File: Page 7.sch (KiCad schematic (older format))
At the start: 7 parts, among them U3 MCP7940N-xSN, Y801 32.7680 kHz

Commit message: Updating Page Numbering
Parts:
- removed R801: 10k0, Resistor_SMD:R_0603_1608Metric_Pad1.05x0.95mm_HandSolder, symbol Device:R
- renumbered C801 to C701, C802 to C702, C803 to C703, Y801 to Y701
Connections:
- wire segments 32 -> 28
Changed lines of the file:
@@
 $Descr A4 11693 8268
 encoding utf-8
-Sheet 9 9
+Sheet 8 9
 Title ""
 Date ""
@@
 AR Path="/5EAC05C2/5EB307E0" Ref="C?"  Part="1"
 AR Path="/5ECF32A9/5EB307E0" Ref="C?"  Part="1"
-AR Path="/5ECF31FF/5EB307E0" Ref="C803"  Part="1"
-F 0 "C803" V 7000 3700 50  0000 C CNN
+AR Path="/5ECF31FF/5EB307E0" Ref="C703"  Part="1"
+F 0 "C703" V 7000 3700 50  0000 C CNN
 F 1 "10pF" V 7300 3700 50  0000 C CNN
 F 2 "Capacitor_SMD:C_0603_1608Metric_Pad1.05x0.95mm_HandSolder" H 7188 3550 50  0001 C CNN
@@
 AR Path="/5EAC05C2/5EB307E8" Ref="C?"  Part="1"
 AR Path="/5ECF32A9/5EB307E8" Ref="C?"  Part="1"
-AR Path="/5ECF31FF/5EB307E8" Ref="C802"  Part="1"
-F 0 "C802" V 7000 4300 50  0000 C CNN
+AR Path="/5ECF31FF/5EB307E8" Ref="C702"  Part="1"
+F 0 "C702" V 7000 4300 50  0000 C CNN
 F 1 "10pF" V 7300 4300 50  0000 C CNN
 F 2 "Capacitor_SMD:C_0603_1608Metric_Pad1.05x0.95mm_HandSolder" H 7188 4150 50  0001 C CNN
@@
 AR Path="/5EAC05C2/5EB307EE" Ref="Y?"  Part="1"
 AR Path="/5ECF32A9/5EB307EE" Ref="Y?"  Part="1"
-AR Path="/5ECF31FF/5EB307EE" Ref="Y801"  Part="1"
-F 0 "Y801" H 6550 3850 50  0000 L CNN
+AR Path="/5ECF31FF/5EB307EE" Ref="Y701"  Part="1"
+F 0 "Y701" H 6550 3850 50  0000 L CNN
 F 1 "32.7680 kHz" H 6400 4150 50  0000 L CNN
 F 2 "Name Plate Class Project:Oscillator_MC-405_32.7680K-D__ROHS" H 6550 3700 50  0001 L BNN
@@
 	-1   0    0    1
 $EndComp
-Wire Wire Line
-	5500 4100 5300 4100
-Text Label 4950 4100 0    50   ~ 0
-RTC_INT
 Text Notes 5300 5050 0    98   ~ 20
 Real Time Clock
-Connection ~ 5300 4100
-Wire Wire Line
-	5300 4100 4950 4100
-$Comp
-L Device:R R?
-U 1 1 5EB30819
-P 5300 3050
-AR Path="/5EAC05C2/5EB30819" Ref="R?"  Part="1"
-AR Path="/5ECF32A9/5EB30819" Ref="R?"  Part="1"
-AR Path="/5ECF31FF/5EB30819" Ref="R801"  Part="1"
-F 0 "R801" H 5370 3096 50  0000 L CNN
-F 1 "10k0" H 5370 3005 50  0000 L CNN
-F 2 "Resistor_SMD:R_0603_1608Metric_Pad1.05x0.95mm_HandSolder" V 5230 3050 50  0001 C CNN
-F 3 "~" H 5300 3050 50  0001 C CNN
-	1    5300 3050
-	1    0    0    -1
-$EndComp
 $Comp
 L Device:C C?
@@
 AR Path="/5EAC05C2/5EB30820" Ref="C?"  Part="1"
 AR Path="/5ECF32A9/5EB30820" Ref="C?"  Part="1"
-AR Path="/5ECF31FF/5EB30820" Ref="C801"  Part="1"
-F 0 "C801" H 4150 3150 50  0000 L CNN
+AR Path="/5ECF31FF/5EB30820" Ref="C701"  Part="1"
+F 0 "C701" H 4150 3150 50  0000 L CNN
 F 1 "0.1uF" H 4150 3050 50  0000 L CNN
 F 2 "Capacitor_SMD:C_0603_1608Metric_Pad1.05x0.95mm_HandSolder" H 4538 2950 50  0001 C CNN
@@
 $EndComp
 Wire Wire Line
-	5300 2900 5300 2800
-Connection ~ 5300 2800
-Wire Wire Line
 	5150 3450 5650 3450
 Wire Wire Line
@@
 Wire Wire Line
 	5900 3600 5900 2800
-Wire Wire Line
-	5300 2800 5900 2800
-Wire Wire Line
-	5300 3200 5300 4100
-Wire Wire Line
-	4500 2800 5300 2800
 Connection ~ 4500 2800
 Wire Wire Line
@@
 Text HLabel 4950 4100 0    50   Input ~ 0
 RTC_INT
+Wire Wire Line
+	4500 2800 5900 2800
+Wire Wire Line
+	4950 4100 5500 4100
 $EndSCHEMATC

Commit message: Updates to schematic
Switching to ATMega34UF chip.
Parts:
- B801: Mftr Part No. (none) -> BK-883
- C701: DigiKey Part No. (none) -> 311-1335-1-ND; Manufacturer (none) -> Yageo; Mftr Part No. Yageo CC0603KPX7R7BB104 -> CC0603KPX7R7BB104
- C702, C703: Manufacturer (none) -> Kemet; Mftr Part No. Kemet C0603C100J1GACTU -> C0603C100J1GACTU
- U701: renamed from U3; DigiKey Part No. (none) -> MCP79400-I/SN-ND; Manufacturer (none) -> Microchip; Mftr Part No. (none) -> MCP79400-I/SN
- Y701: DigiKey Part No. (none) -> SER4311TR-ND; Manufacturer (none) -> Epson; Mftr Part No. (none) -> MC-405 32.7680K-E3: ROHS
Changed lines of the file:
@@
 F 1 "10pF" V 7300 3700 50  0000 C CNN
 F 2 "Capacitor_SMD:C_0603_1608Metric_Pad1.05x0.95mm_HandSolder" H 7188 3550 50  0001 C CNN
-F 3 "~" H 7150 3700 50  0001 C CNN
+F 3 "https://content.kemet.com/datasheets/KEM_C1003_C0G_SMD.pdf" H 7150 3700 50  0001 C CNN
 F 4 "399-7816-1-ND" H 7150 3700 50  0001 C CNN "DigiKey Part No."
-F 5 "Kemet C0603C100J1GACTU" H 7150 3700 50  0001 C CNN "Mftr Part No."
+F 5 "C0603C100J1GACTU" H 7150 3700 50  0001 C CNN "Mftr Part No."
+F 6 "Kemet" H 7150 3700 50  0001 C CNN "Manufacturer"
 	1    7150 3700
 	0    1    1    0
@@
 F 1 "10pF" V 7300 4300 50  0000 C CNN
 F 2 "Capacitor_SMD:C_0603_1608Metric_Pad1.05x0.95mm_HandSolder" H 7188 4150 50  0001 C CNN
-F 3 "~" H 7150 4300 50  0001 C CNN
+F 3 "https://content.kemet.com/datasheets/KEM_C1003_C0G_SMD.pdf" H 7150 4300 50  0001 C CNN
 F 4 "399-7816-1-ND" H 7150 4300 50  0001 C CNN "DigiKey Part No."
-F 5 "Kemet C0603C100J1GACTU" H 7150 4300 50  0001 C CNN "Mftr Part No."
+F 5 "C0603C100J1GACTU" H 7150 4300 50  0001 C CNN "Mftr Part No."
+F 6 "Kemet" H 7150 4300 50  0001 C CNN "Manufacturer"
 	1    7150 4300
 	0    1    1    0
@@
 F 2 "Name Plate Class Project:Oscillator_MC-405_32.7680K-D__ROHS" H 6550 3700 50  0001 L BNN
 F 3 "https://support.epson.biz/td/api/doc_check.php?dl=brief_MC-405&lang=en" H 6550 3600 50  0001 L BNN
+F 4 "SER4311TR-ND" H 6650 4000 50  0001 C CNN "DigiKey Part No."
+F 5 "Epson " H 6650 4000 50  0001 C CNN "Manufacturer"
+F 6 "MC-405 32.7680K-E3: ROHS" H 6650 4000 50  0001 C CNN "Mftr Part No."
 	1    6650 4000
 	0    1    1    0
@@
 F 4 "MPD" H 4700 3150 50  0001 L BNN "Field4"
 F 5 "L" H 4700 3050 50  0001 L BNN "Field5"
-F 6 "" H 4850 3450 50  0001 C CNN "Mftr Part No."
+F 6 "BK-883" H 4850 3450 50  0001 C CNN "Mftr Part No."
 F 7 "BK-883-ND" H 4850 3450 50  0001 C CNN "DigiKey Part No."
 F 8 "MPD" H 4850 3450 50  0001 C CNN "Manufacturer"
@@
 F 2 "Capacitor_SMD:C_0603_1608Metric_Pad1.05x0.95mm_HandSolder" H 4538 2950 50  0001 C CNN
 F 3 "https://www.yageo.com/upload/media/product/productsearch/datasheet/mlcc/UPY-GPHC_X7R_6.3V-to-50V_18.pdf" H 4500 3100 50  0001 C CNN
-F 4 "Yageo CC0603KPX7R7BB104" H 4500 3100 50  0001 C CNN "Mftr Part No."
+F 4 "CC0603KPX7R7BB104" H 4500 3100 50  0001 C CNN "Mftr Part No."
+F 5 "Yageo" H 4500 3100 50  0001 C CNN "Manufacturer"
+F 6 "311-1335-1-ND" H 4500 3100 50  0001 C CNN "DigiKey Part No."
 	1    4500 3100
 	1    0    0    -1
@@
 AR Path="/5EAC05C2/5EB307D8" Ref="U?"  Part="1"
 AR Path="/5ECF32A9/5EB307D8" Ref="U?"  Part="1"
-AR Path="/5ECF31FF/5EB307D8" Ref="U3"  Part="1"
-F 0 "U3" H 6000 3600 50  0000 L BNN
+AR Path="/5ECF31FF/5EB307D8" Ref="U701"  Part="1"
+F 0 "U701" H 6000 3600 50  0000 L BNN
 F 1 "MCP7940N-xSN" H 6000 3500 50  0000 L BNN
 F 2 "Package_SO:SOIC-8_3.9x4.9mm_P1.27mm" H 5900 4000 50  0001 C CNN
 F 3 "http://ww1.microchip.com/downloads/en/DeviceDoc/20005010F.pdf" H 5900 4000 50  0001 C CNN
+F 4 "MCP79400-I/SN-ND" H 5900 4000 50  0001 C CNN "DigiKey Part No."
+F 5 "Microchip" H 5900 4000 50  0001 C CNN "Manufacturer"
+F 6 "MCP79400-I/SN" H 5900 4000 50  0001 C CNN "Mftr Part No."
 	1    5900 4000
 	1    0    0    -1

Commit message: Updates
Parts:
- B701: renamed from B801; footprint Name Plate Class Project:BAT_BK-883 -> Name_Plate_Class_Project:BAT_BK-883; symbol Name~Plate~Class~Library:BK-883 -> Name_Plate_Class_Project:BK-883; Field4 MPD -> (none); Field5 L -> (none)
- Y701: footprint Name Plate Class Project:Oscillator_MC-405_32.7680K-D__ROHS -> Name_Plate_Class_Project:Oscillator_MC-405_32.7680K-D__ROHS; symbol Name~Plate~Class~Library:Oscillator_MC-405_32.7680K-D__ROHS -> Name_Plate_Class_Project:Oscillator_MC-405_32.7680K-D__ROHS
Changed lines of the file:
@@
 $EndComp
 $Comp
-L Name~Plate~Class~Library:Oscillator_MC-405_32.7680K-D__ROHS Y?
+L Name_Plate_Class_Project:Oscillator_MC-405_32.7680K-D__ROHS Y?
 U 1 1 5EB307EE
 P 6650 4000
@@
 F 0 "Y701" H 6550 3850 50  0000 L CNN
 F 1 "32.7680 kHz" H 6400 4150 50  0000 L CNN
-F 2 "Name Plate Class Project:Oscillator_MC-405_32.7680K-D__ROHS" H 6550 3700 50  0001 L BNN
+F 2 "Name_Plate_Class_Project:Oscillator_MC-405_32.7680K-D__ROHS" H 6550 3700 50  0001 L BNN
 F 3 "https://support.epson.biz/td/api/doc_check.php?dl=brief_MC-405&lang=en" H 6550 3600 50  0001 L BNN
 F 4 "SER4311TR-ND" H 6650 4000 50  0001 C CNN "DigiKey Part No."
@@
 $EndComp
 $Comp
-L Name~Plate~Class~Library:BK-883 B?
+L Name_Plate_Class_Project:BK-883 B?
 U 1 1 5EB3080E
 P 4850 3450
 AR Path="/5EAC05C2/5EB3080E" Ref="B?"  Part="1"
 AR Path="/5ECF32A9/5EB3080E" Ref="B?"  Part="1"
-AR Path="/5ECF31FF/5EB3080E" Ref="B801"  Part="1"
-F 0 "B801" H 4850 3183 50  0000 C CNN
+AR Path="/5ECF31FF/5EB3080E" Ref="B701"  Part="1"
+F 0 "B701" H 4850 3183 50  0000 C CNN
 F 1 "BK-883" H 4850 3274 50  0000 C CNN
-F 2 "Name Plate Class Project:BAT_BK-883" H 4700 3700 50  0001 L BNN
+F 2 "Name_Plate_Class_Project:BAT_BK-883" H 4700 3700 50  0001 L BNN
 F 3 "https://www.memoryprotectiondevices.com/datasheets/BK-883-datasheet.pdf" H 4700 3100 50  0001 L BNN
-F 4 "MPD" H 4700 3150 50  0001 L BNN "Field4"
-F 5 "L" H 4700 3050 50  0001 L BNN "Field5"
-F 6 "BK-883" H 4850 3450 50  0001 C CNN "Mftr Part No."
-F 7 "BK-883-ND" H 4850 3450 50  0001 C CNN "DigiKey Part No."
-F 8 "MPD" H 4850 3450 50  0001 C CNN "Manufacturer"
+F 4 "BK-883" H 4850 3450 50  0001 C CNN "Mftr Part No."
+F 5 "BK-883-ND" H 4850 3450 50  0001 C CNN "DigiKey Part No."
+F 6 "MPD" H 4850 3450 50  0001 C CNN "Manufacturer"
 	1    4850 3450
 	-1   0    0    1

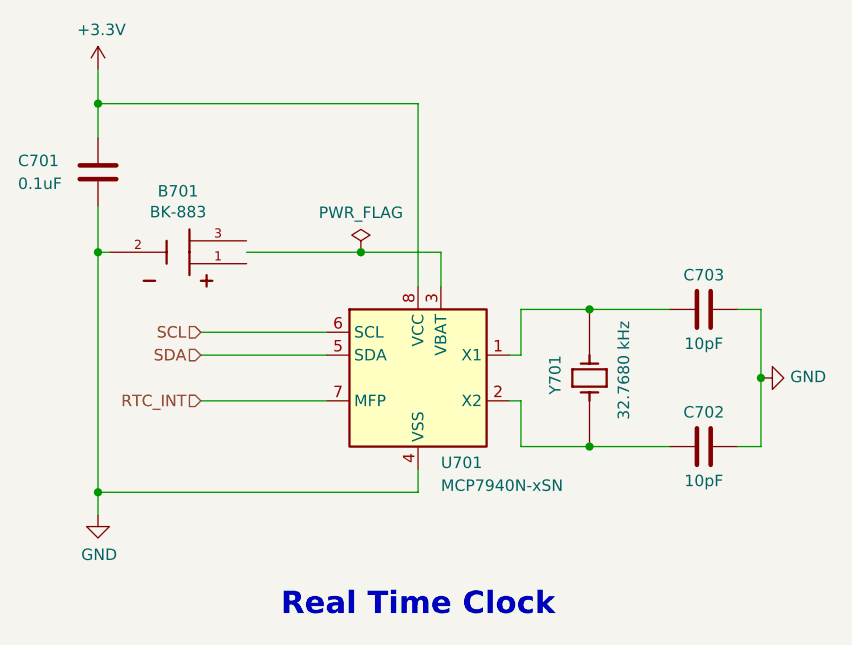
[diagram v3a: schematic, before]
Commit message: PCB Update
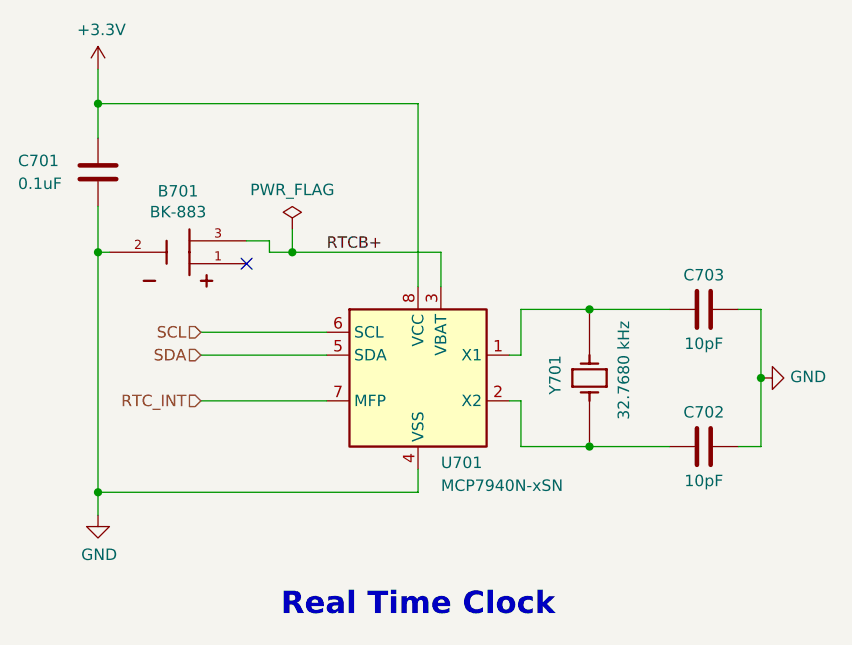
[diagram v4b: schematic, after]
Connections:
- net labels added: RTCB+
- wire segments 28 -> 31
- no-connect marks 0 -> 1
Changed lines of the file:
@@
 $EndComp
 Wire Wire Line
-	5150 3450 5650 3450
+	5250 3450 5350 3450
 Wire Wire Line
 	6000 3450 6000 3600
@@
 L power:PWR_FLAG #FLG0101
 U 1 1 5ED8645E
-P 5650 3450
-F 0 "#FLG0101" H 5650 3525 50  0001 C CNN
-F 1 "PWR_FLAG" H 5650 3623 50  0000 C CNN
-F 2 "" H 5650 3450 50  0001 C CNN
-F 3 "~" H 5650 3450 50  0001 C CNN
-	1    5650 3450
+P 5350 3350
+F 0 "#FLG0101" H 5350 3425 50  0001 C CNN
+F 1 "PWR_FLAG" H 5350 3523 50  0000 C CNN
+F 2 "" H 5350 3350 50  0001 C CNN
+F 3 "~" H 5350 3350 50  0001 C CNN
+	1    5350 3350
 	1    0    0    -1
 $EndComp
-Connection ~ 5650 3450
+Connection ~ 5350 3450
 Wire Wire Line
-	5650 3450 6000 3450
+	5350 3450 6000 3450
 Wire Wire Line
 	4500 3450 4500 4500
@@
 Wire Wire Line
 	4950 4100 5500 4100
+Wire Wire Line
+	5350 3350 5350 3450
+Text Label 5500 3450 0    50   ~ 0
+RTCB+
+NoConn ~ 5150 3500
+Wire Wire Line
+	5150 3400 5250 3400
+Wire Wire Line
+	5250 3400 5250 3450
 $EndSCHEMATC
